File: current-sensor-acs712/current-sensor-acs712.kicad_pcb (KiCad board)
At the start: 2 copper layers, 29 parts, among them J1 Conn_01x02, J2 Conn_01x02, J3 Conn_01x08, U1 ACS712xLCTR-20A, U2 Opamp_Dual

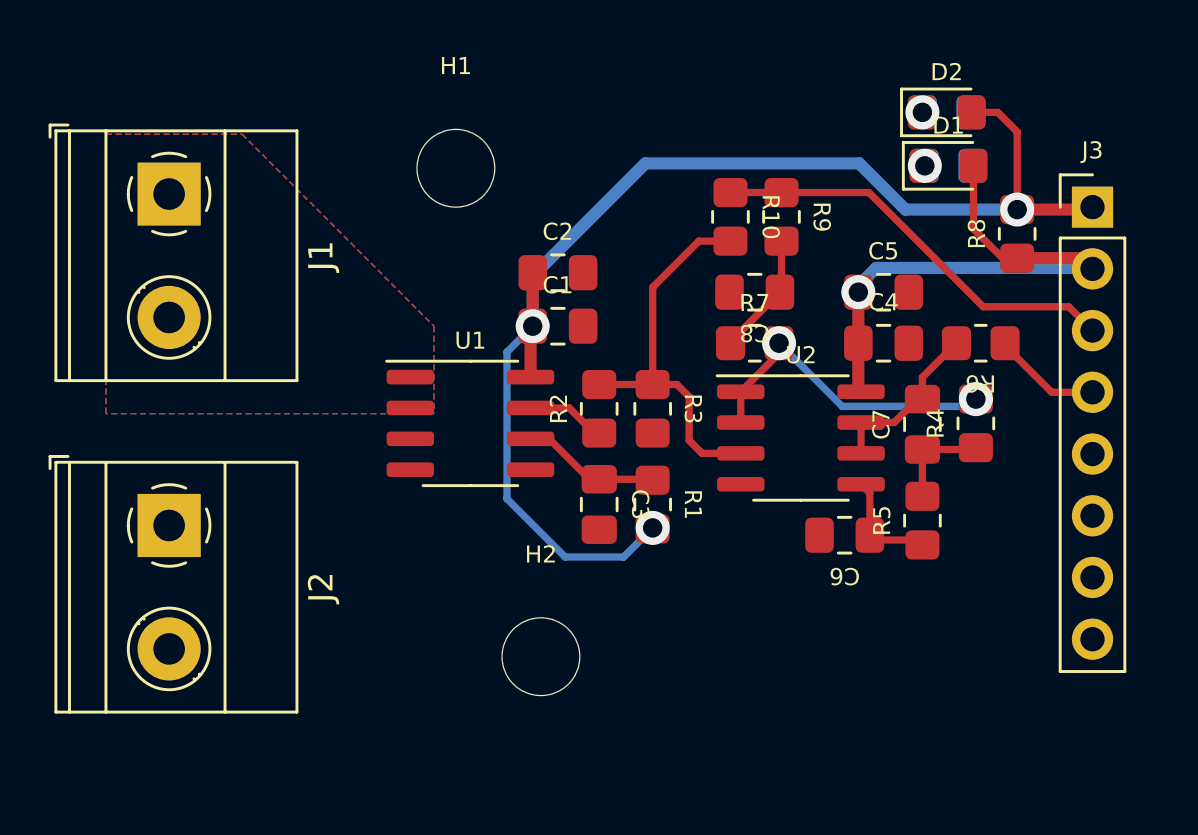
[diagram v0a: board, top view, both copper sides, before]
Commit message: Finishing acs712 board
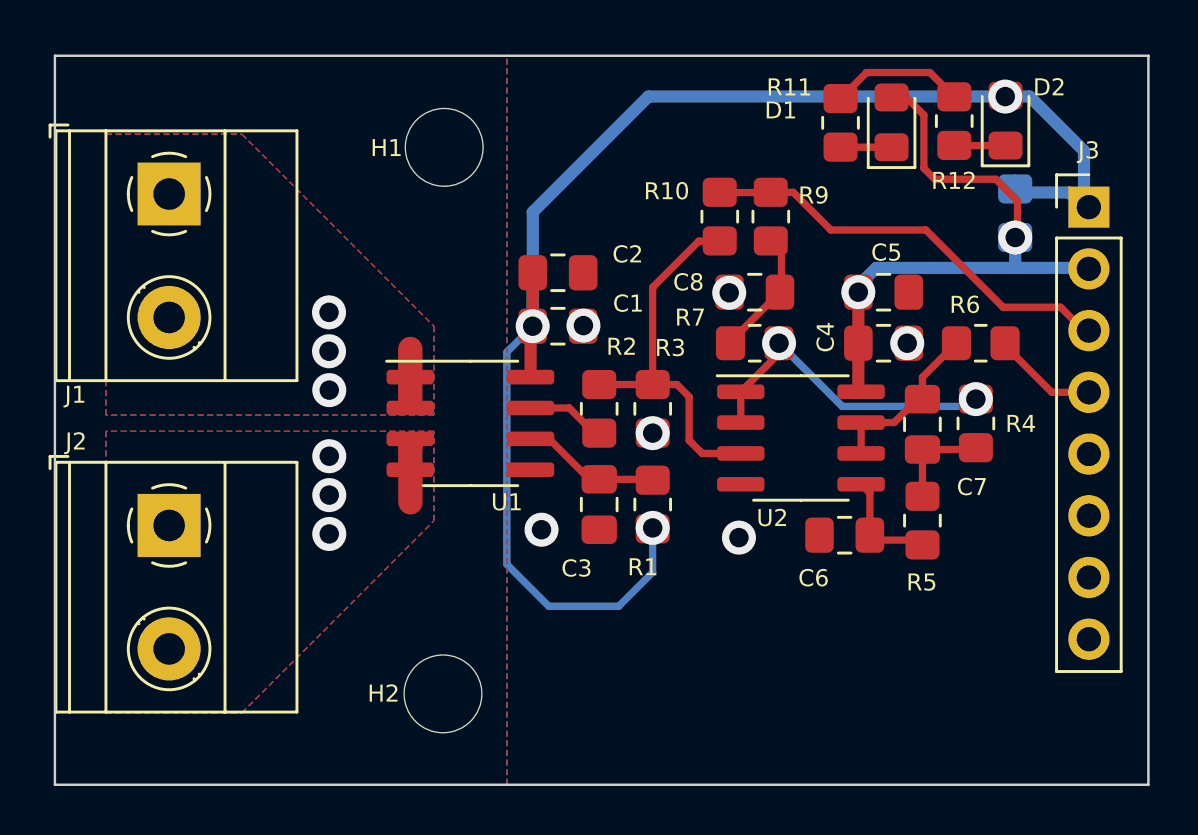
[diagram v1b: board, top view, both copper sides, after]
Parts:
- R11, R12: moved to F.Cu
- R8: moved to B.Cu
- moved R11 4.78 mm to (104.8, 43.8), turned to 90 degrees
- moved H2 4.31 mm to (88.5, 67.3)
- moved D1 2.95 mm to (106.9, 43.8), turned to 90 degrees
- moved D2 2.44 mm to (111.6, 43.7), turned to 90 degrees
- moved H1 0.98 mm to (88.5, 44.8)
- moved R8 0.85 mm to (112.0, 47.5)
- moved R12 0.48 mm to (109.5, 43.8), turned to 90 degrees
- moved R9 0.44 mm to (102.0, 47.7)
- moved R10 0.44 mm to (99.9, 47.7)
- moved J3 0.15 mm to (115.0, 47.3)
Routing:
- net VDD: track 52.6 -> 59.9 mm
- net GND: track 0.00 -> 5.54 mm, vias 0 -> 6
- net VCC: track 22.7 -> 25.4 mm, vias 1 -> 2
- net /I-: track 0.00 -> 2.31 mm, vias 0 -> 3
- net Net-(D2-Pad1): track 0.00 -> 2.11 mm, vias 1 -> 0
- net Net-(D1-Pad1): track 0.00 -> 2.10 mm, vias 1 -> 0
- net /I+: track 0.00 -> 2.09 mm, vias 0 -> 3
- added copper zone on B.Cu, net /I-
- added copper zone on F.Cu, net /I-
- added copper zone on B.Cu, net GND
- added copper zone on F.Cu, net GND
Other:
- board outline added: 45 x 30 mm
